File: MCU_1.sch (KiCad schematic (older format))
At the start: 18 parts, among them U2 STM32F051K6Ux

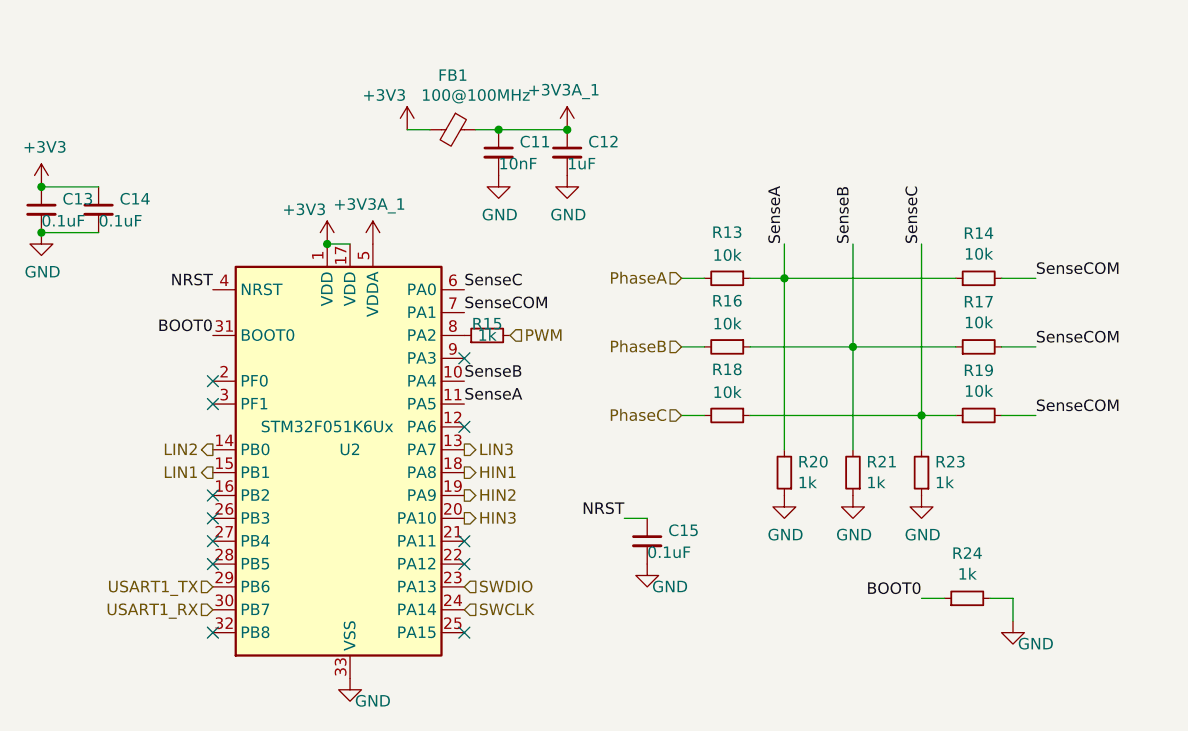
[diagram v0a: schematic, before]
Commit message: Added stuff
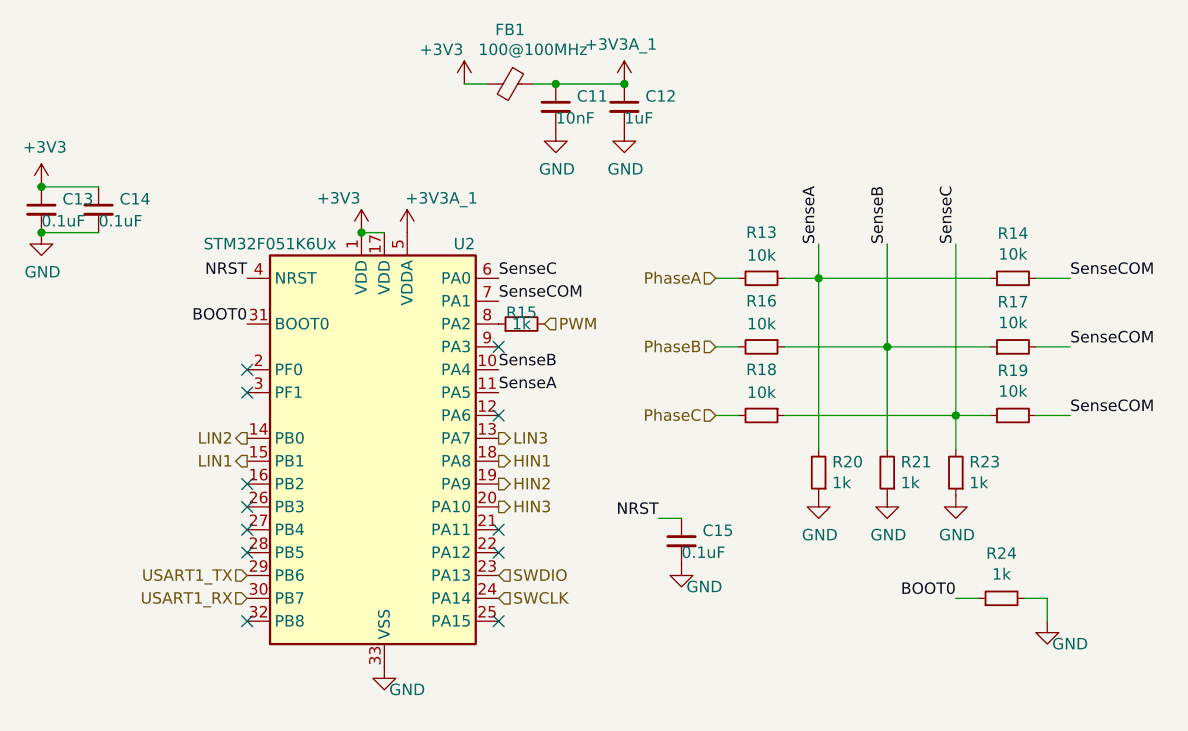
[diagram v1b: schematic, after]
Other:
- moved on the sheet: C11, C12, C15, FB1, R13, R14, R15, R16, R17, R18, R19, R20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
